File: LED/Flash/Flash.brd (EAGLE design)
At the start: 29.2 x 17.8 mm, 14 parts

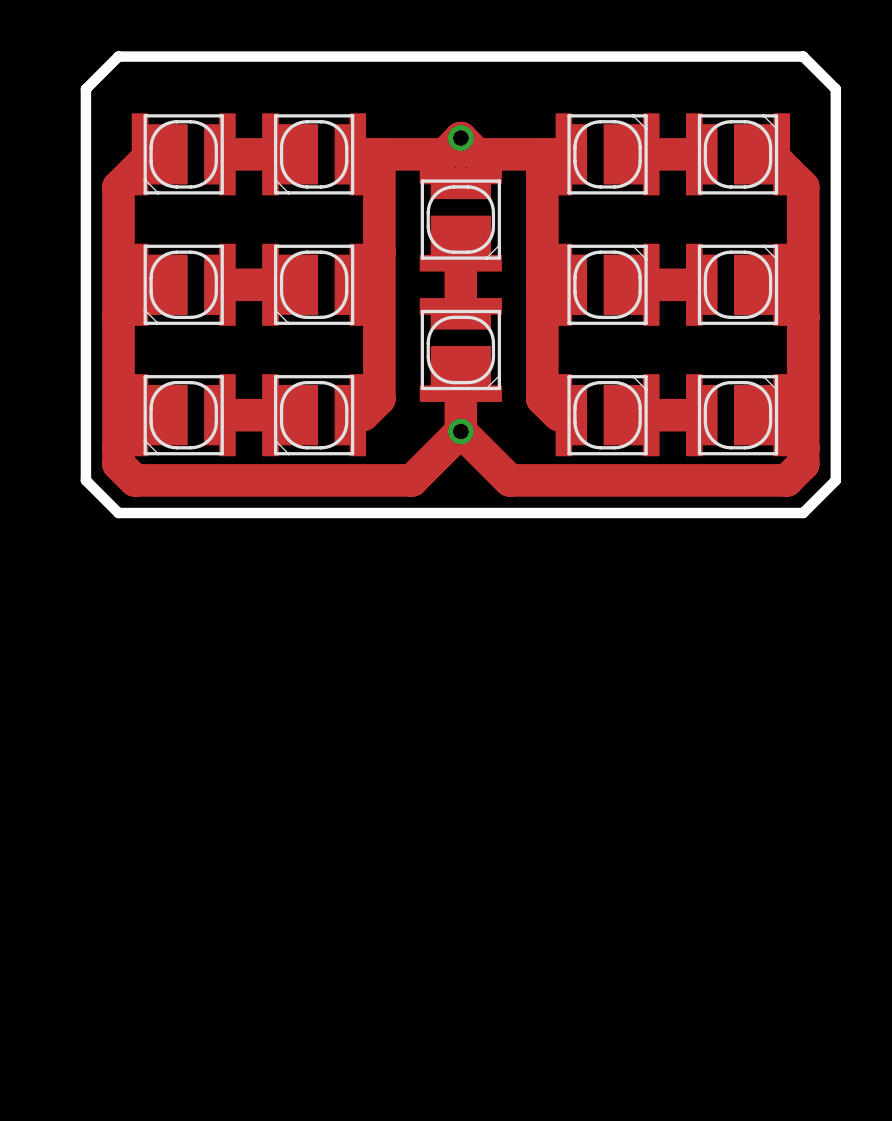
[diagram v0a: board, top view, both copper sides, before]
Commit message: More Flash
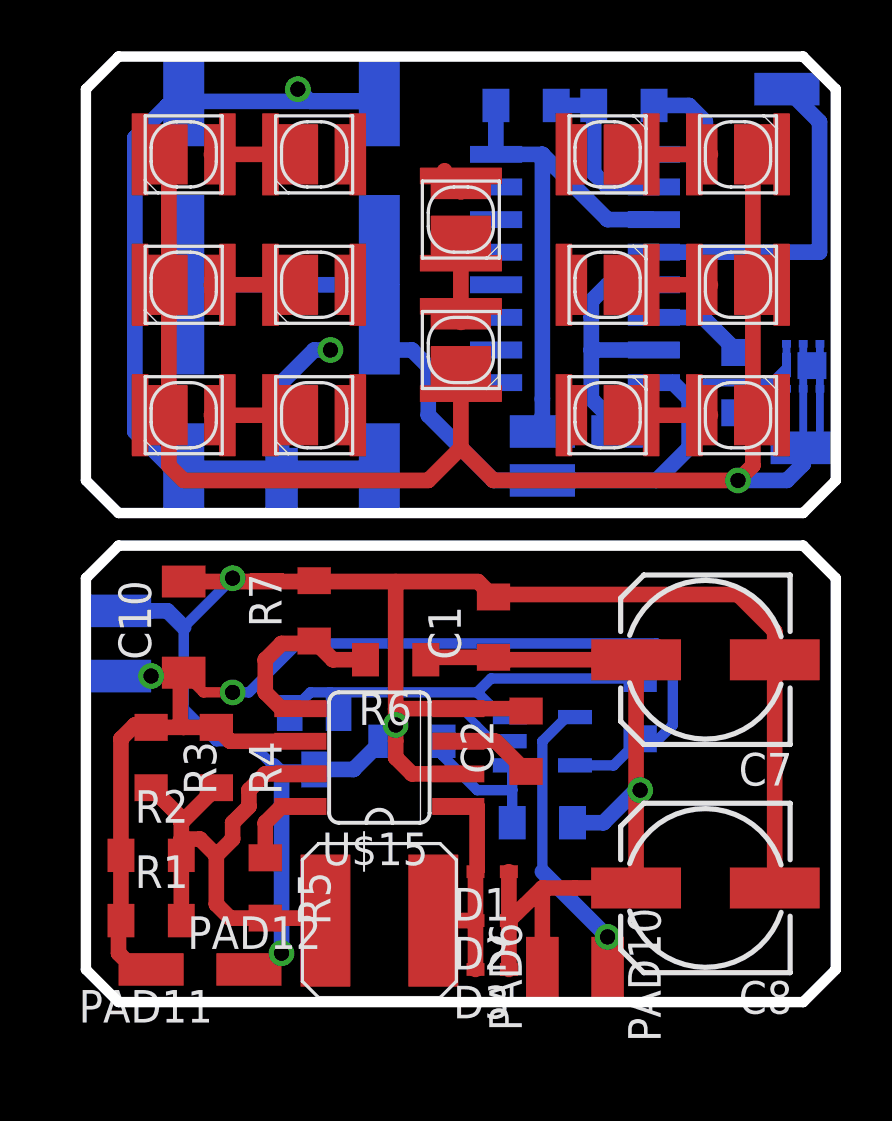
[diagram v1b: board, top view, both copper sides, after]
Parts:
- added C1: 0u1, rcl:C0805
- added C10: 10u, rcl:C1206
- added C2: 1n5, rcl:C0805
- added C3, C4, C5, C6, C7, C8: 47u16v, rcl:153CLV-0605
- added C9: 10u, rcl:C0805
- added D1, D2, D3: RB520S30T1G, diode:SOD523
- added IC1: 4098D, 40xx:SO16
- added PAD1, PAD10, PAD11, PAD12, PAD2, PAD3, PAD4, PAD5, PAD6, PAD7, PAD8, PAD9: (no value), wirepad:SMD1,27-2,54
- added R1, R2, R3, R4: 1R, rcl:R0805
- added R10: 1K, rcl:R0805
- added R11: 43K, rcl:R0805
- added R12: 11K, rcl:R0805
- added R5: 180R, rcl:R0805
- added R6: 12K, rcl:R0805
- added R7: 1K3, rcl:R0805
- added R8: 1M, rcl:R0805
- added R9: 0R, rcl:R0805
- added TL1: TL431CDBZR, Namenlos:SOT23
- added U$15: MC33063/MC34063D, Namenlos at:SO08
- added U$16: 150uH, Namenlos:L6045
- added U$17: STL6N3LLH6, Namenlos:POWERFLAT-2X2
- added U1: TSV621ILT, ST Microelctronics_By_element14_Batch_1:SOT95P280X145-5N
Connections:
- new net +12V: C1.1, C3.+, C4.+, C5.+, C6.+, C7.+, C8.+, D1.C, D2.C, D3.C, PAD6.1, PAD9.1, R11.1, R6.1, U$1.P$1, U$11.P$1, U$13.P$1, U$3.P$1, U$5.P$1, U$7.P$1, U$9.P$1
- new net B+: C10.1, IC1.16, IC1.3, PAD1.1, PAD11.1, PAD8.1, R1.1, R10.1, R2.1, R3.1, R4.1, R8.2, U$15.6, U1.5
- new net GND: C1.2, C10.2, C2.2, C3.-, C4.-, C5.-, C6.-, C7.-, C8.-, IC1.8, PAD12.1, PAD2.1, PAD7.1, R12.2, R7.2, TL1.3, U$15.2, U$15.4, U$17.S, U$17.S4, U1.2
- new net N$11: R6.2, R7.1, U$15.5
- new net N$12: D1.A, D2.A, D3.A, U$15.1, U$16.P$2
- new net N$14: C2.1, U$15.3
- new net N$17: C9.2, IC1.1
- new net N$18: C9.1, IC1.2, R8.1
- new net N$20: IC1.6, R9.2
- new net N$21: R9.1, U$17.G3
- new net N$5: R11.2, R12.1, U1.1
- new net N$6: IC1.4, PAD3.1
- new net N$8: R1.2, R2.2, R3.2, R4.2, R5.2, U$15.7, U$16.P$1
- new net N$9: R5.1, U$15.8
- new net TR-: IC1.5, IC1.7, PAD10.1, PAD4.1, U1.4
- net N$2: now also R10.2, TL1.1, TL1.2, U1.3; no longer U$1.P$1, U$11.P$1, U$13.P$1, U$3.P$1, U$5.P$1, U$7.P$1, U$9.P$1
- net N$3: now also PAD5.1, U$17.D, U$17.D1, U$17.D2, U$17.D5, U$17.D6
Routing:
- net GND: track 0.00 -> 127.3 mm, vias 0 -> 3
- net +12V: track 0.00 -> 75.5 mm, vias 0 -> 3
- net B+: track 0.00 -> 69.7 mm, vias 0 -> 2
- net TR-: track 0.00 -> 22.3 mm, vias 0 -> 1
- net N$2: track 38.1 -> 16.8 mm, vias 1 -> 0
- net N$8: track 0.00 -> 21.0 mm
- net N$6: track 0.00 -> 13.3 mm
- net N$12: track 0.00 -> 8.76 mm
- net N$11: track 0.00 -> 7.41 mm
- net N$18: track 0.00 -> 6.66 mm
- net N$5: track 0.00 -> 6.11 mm
- net N$17: track 0.00 -> 5.17 mm
- net N$20: track 0.00 -> 3.84 mm
- net N$3: track 67.9 -> 64.3 mm
- net N$14: track 0.00 -> 3.13 mm
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- added copper zone on layer 1, net +12V
- removed copper zone on layer 1, net N$2
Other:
- board size 29.2 x 17.8 mm -> 29.2 x 36.8 mm
